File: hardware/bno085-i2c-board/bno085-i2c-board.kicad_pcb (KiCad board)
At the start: 2 copper layers, 8 parts, among them J1 Conn_01x06_Pin

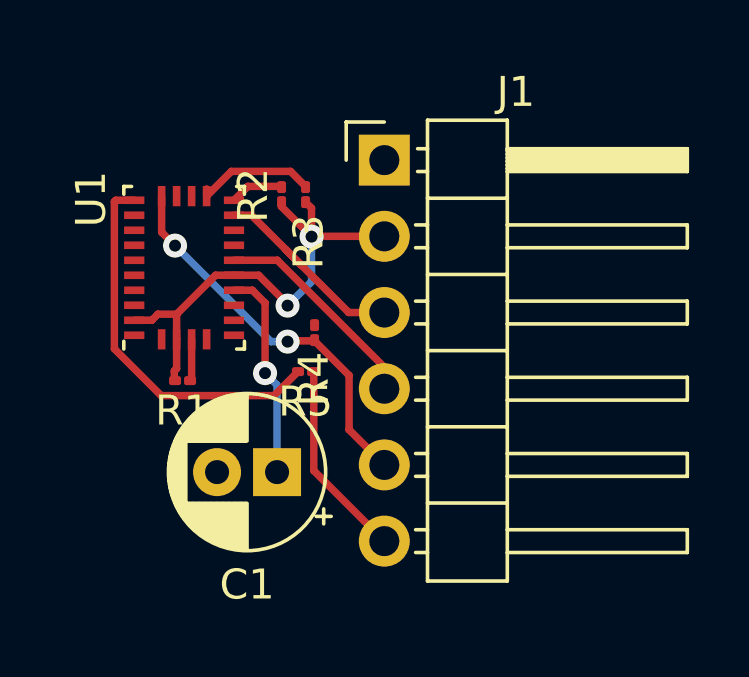
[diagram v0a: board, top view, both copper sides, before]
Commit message: more pcb
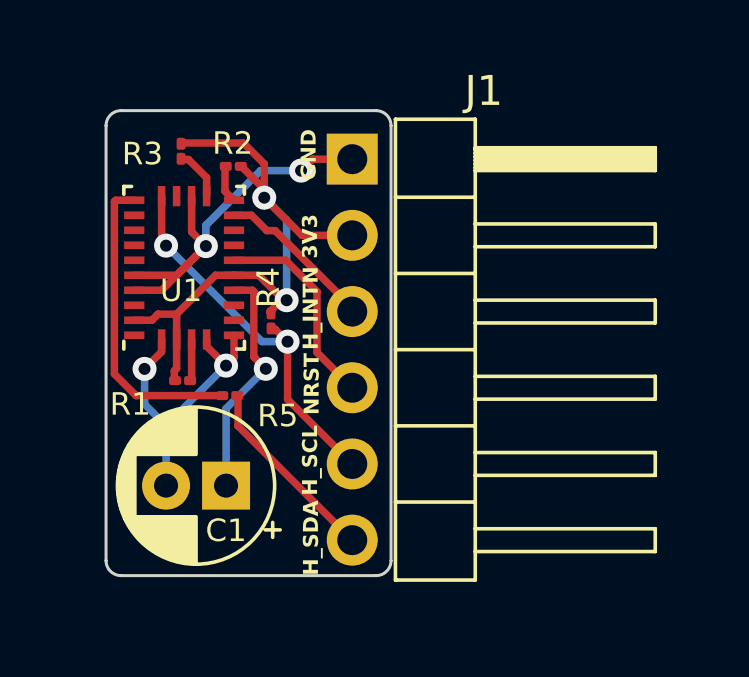
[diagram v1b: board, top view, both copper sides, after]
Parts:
- moved R3 4.39 mm to (156.5, 83.4), turned to 90 degrees
- moved R5 2.65 mm to (158.1, 91.5)
- moved R2 1.86 mm to (158.2, 83.9), turned to 180 degrees
- moved C1 1.76 mm to (158.0, 94.5)
- moved R4 1.50 mm to (159.5, 89.0)
- moved J1 1.07 mm to (162.2, 83.6)
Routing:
- net GND: track 0.00 -> 24.6 mm, vias 0 -> 4
- net +3.3V: track 16.4 -> 21.9 mm
- net Net-(U1-H_SDA/H_MISO/TX): track 12.7 -> 10.3 mm
- net Net-(U1-ENV_SDA): track 4.09 -> 1.72 mm
- net /H_INTN: track 7.10 -> 5.35 mm
- net Net-(U1-CAP): track 7.02 -> 7.86 mm
- net Net-(U1-ENV_SCL): track 1.78 -> 1.25 mm
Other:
- board outline added: 9.5 x 15.5 mm
- board text added: "3V3"
- board text added: "GND"
- board text added: "H_INTN"
- board text added: "H_SCL"
- board text added: "H_SDA"
- board text added: "NRST"
